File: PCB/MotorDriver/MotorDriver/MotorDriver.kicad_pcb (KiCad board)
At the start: 2 copper layers, 101.3 x 73.7 mm, 93 parts, among them J1 XT30PW-M, J10 JST-XH, J11 JST-XH, J12 JST-XH, J13 JST-XH, J14 JST-XH, J15 JST-XH, J16 JST-XH, J17 JST-XH, J18 JST-XH, J19 JST-XH, J2 JST-XH, J20 JST-XH, J21 JST-XH, J22 JST-XH, J23 JST-XH, J24 JST-XH, J3 XT30PW-M, J4 XT30PW-M, J5 JST-XH, J6 JST-XH, J7 JST-XH, J8 JST-XH, J9 JST-XH, Q1 TJ60S04M3L, Q10 NMOS, Q2 NMOS, Q3 NMOS, Q4 NMOS, Q5 NMOS, Q6 NMOS, Q7 NMOS, Q8 NMOS, Q9 NMOS, SW1 SW_DPST_x2, SW2 SW_Push, SW3 SW_Push, U1 DRV8701ERGET, U2 DRV8701ERGET, U3 TCA9548APWR, U4 Pico, U5 AZ1117CH-3.3TR

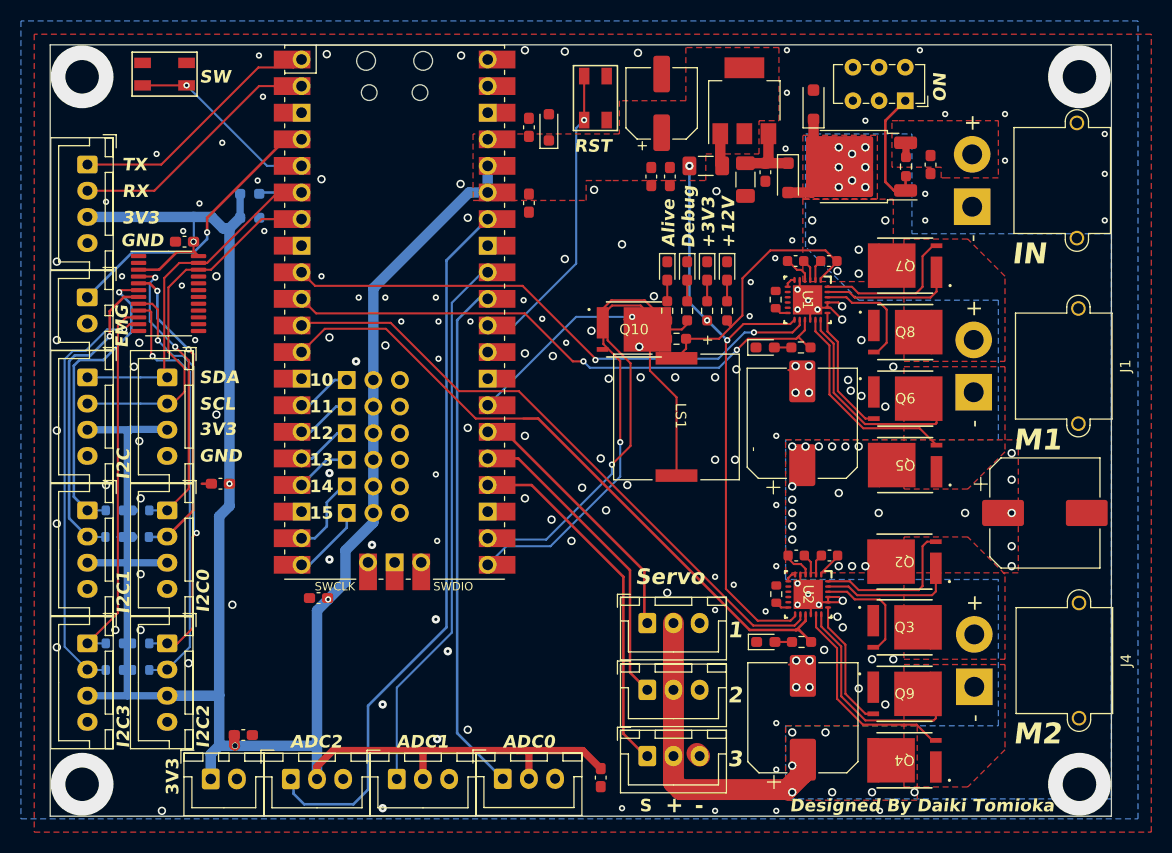
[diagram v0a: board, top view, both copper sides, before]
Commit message: ✏️ 昔のファイルを引っ張てきた
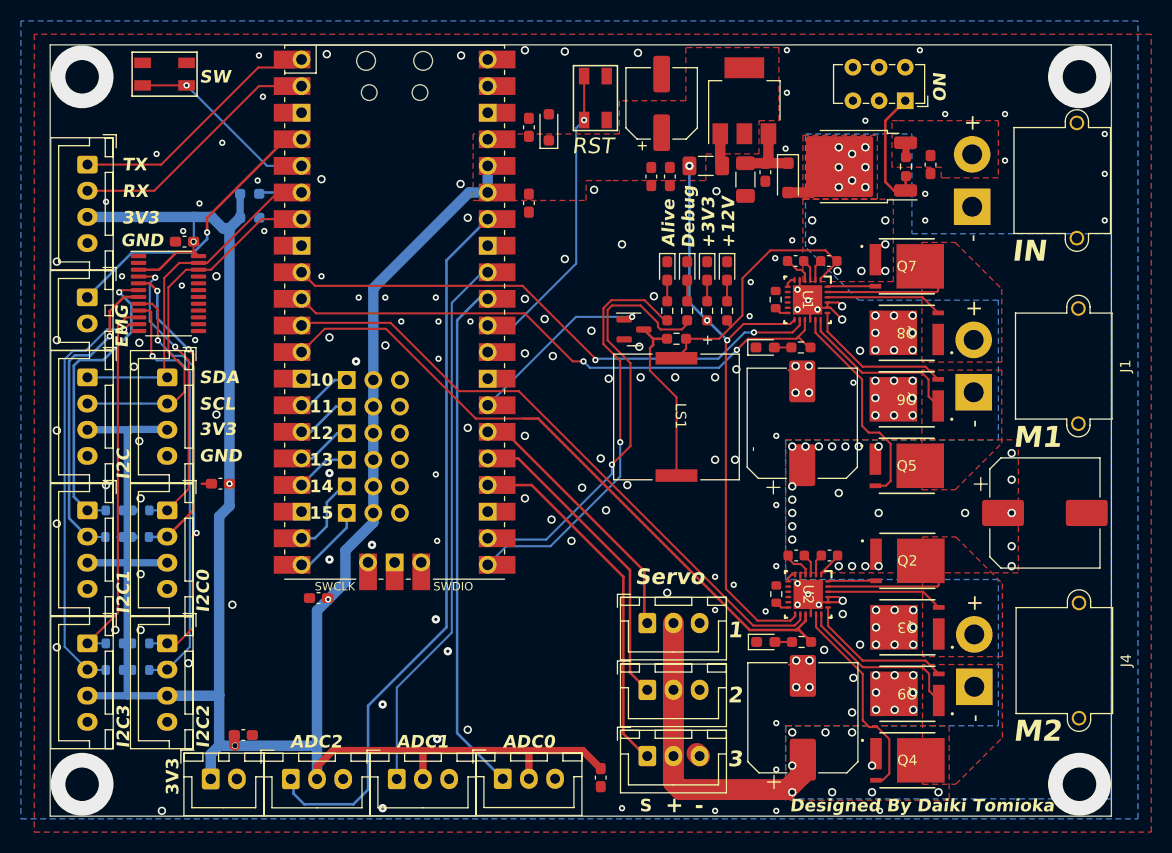
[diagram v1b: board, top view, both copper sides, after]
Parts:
- removed D2: ＧＳ１０１０ＦＬ, Diode_SMD:D_SOD-123F
- Q10: footprint TPH11006NL:TPH11006NL_SOP Advance_TOS-M -> Package_TO_SOT_SMD:SOT-23
- moved Q2 0.29 mm to (132.9, 148.1), turned to 0 degrees
- moved Q4 0.28 mm to (132.9, 167.1), turned to 0 degrees
- moved Q3 0.27 mm to (132.9, 154.4), turned to 180 degrees
- moved Q9 0.27 mm to (132.9, 160.8), turned to 180 degrees
- moved Q7 0.17 mm to (132.9, 120.0), turned to 0 degrees
- moved Q5 0.17 mm to (132.9, 139.0), turned to 0 degrees
- moved Q6 0.16 mm to (132.9, 132.7), turned to 180 degrees
- moved Q8 0.16 mm to (132.9, 126.3), turned to 180 degrees
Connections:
- R2 pad 2: GND -> Net-(Q1-G)
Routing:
- net GND: track 44.7 -> 32.4 mm, vias 155 -> 180
- net Net-(Q1-G): track 0.00 -> 12.3 mm
- net Net-(Q2-G): track 14.9 -> 4.60 mm
- net Net-(Q7-G): track 14.3 -> 4.60 mm
- net +12V: track 68.8 -> 65.1 mm, vias 43 -> 48
- net Motor2A: track 21.0 -> 17.6 mm
- net Motor1A: track 20.9 -> 17.6 mm
- net Motor1B: track 12.7 -> 15.0 mm
- net Motor2B: track 13.0 -> 15.0 mm
- net Net-(Q9-G): track 12.4 -> 14.2 mm
- net Net-(Q6-G): track 12.4 -> 14.2 mm
- net Net-(Q5-G): track 19.9 -> 20.6 mm
- net Net-(Q3-G): track 10.7 -> 11.3 mm
